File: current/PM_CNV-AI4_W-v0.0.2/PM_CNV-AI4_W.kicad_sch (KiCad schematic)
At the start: 71 parts, among them J1 AFA07-S10FCC-00, J4 15EDGRHC-THR-3.5-14P, J5 15EDGRHC-THR-3.5-14P, U1 AD7190BRUZ, U2 AD7190BRUZ, U3 CA-IS3761HW, U4 CA-IS3105W

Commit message: PM_CNV-AI4_W-v0.0.2
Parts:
- removed C10, C4: 10 uF, kicad_inventree_lib:TAJA_AVX-M, symbol kicad_inventree_lib:TAJA106M016RNJ
- removed C12, C37: 10uF, Capacitor_SMD:C_0603_1608Metric, symbol kicad_inventree_lib:C_10uF_16V_0603_MLCC-X5R
- removed C2, C8: 100nF, Capacitor_SMD:C_0603_1608Metric, symbol kicad_inventree_lib:C_100nF_16V_0603_MLCC-X7R
- removed C22, C24, C31, C33, C34, C36: 10nF, Capacitor_SMD:C_0603_1608Metric, symbol kicad_inventree_lib:C_10nF_16V_0603_MLCC-X7R
- removed C23, C32, C35: 1uF, Capacitor_SMD:C_0603_1608Metric, symbol kicad_inventree_lib: C_1uF_16V_0603_MLCC-X7R
- removed J1: AFA07-S10FCC-00, kicad_inventree_lib:CONN10_AFA07-S10_JUS, symbol kicad_inventree_lib:AFA07-S10FCC-00
- removed JP5, JP6, JP7, JP8: SolderJumper_2_Open, Jumper:SolderJumper-2_P1.3mm_Open_RoundedPad1.0x1.5mm, symbol Jumper:SolderJumper_2_Open
- removed R10: 10k, Resistor_SMD:R_0603_1608Metric, symbol kicad_inventree_lib:R_10k_0603_1%
- removed U1, U2: AD7190BRUZ, kicad_inventree_lib:RU_24_ADI-M, symbol kicad_inventree_lib:AD7190BRUZ
- removed U3: CA-IS3761HW, kicad_inventree_lib:SOIC16-WBW_CLG-M, symbol kicad_inventree_lib:CA-IS3761HW
- added C12, C37: 10uF, Capacitor_SMD:C_0805_2012Metric, symbol kicad_inventree_lib:C_10uF_16V_0805_MLCC-X7R
- added D1, D2, D3: XL-1606SYGC, kicad_inventree_lib:XL-1606, symbol kicad_inventree_lib:XL-1606SYGC
- added D17, D18: XL-1606UBC, kicad_inventree_lib:XL-1606, symbol kicad_inventree_lib:XL-1606UBC
- added D4, D5: XL-1606SURC, kicad_inventree_lib:XL-1606, symbol kicad_inventree_lib:XL-1606SURC
- added J1: FFC_12P_P1.0_100mm_straight, symbol kicad_inventree_lib:FFC_12P_P1.0_100mm_straight
- added J2, J6, J7: AFA07-S12FCC-00, kicad_inventree_lib:CONN10_AFA07-S12_JUS, symbol kicad_inventree_lib:AFA07-S12FCC-00
- added J3: FFC_10P_P1.0_50mm_reverse, symbol kicad_inventree_lib:FFC_10P_P1.0_50mm_reverse
- added R10, R12, R13, R14, R15, R16, R17: 1k, Resistor_SMD:R_0603_1608Metric, symbol kicad_inventree_lib:R_1k_0603_1%
- added SP1: ~, kicad_inventree_lib:PM_LED-xx-v0.0.1, symbol kicad_inventree_lib:PM_LED-10-v0.0.1
- added U1, U2: 5117, kicad_inventree_lib:5117, symbol kicad_inventree_lib:5117
- added U5: SN74LVC2G14DBVR, kicad_inventree_lib:DBV6-M, symbol kicad_inventree_lib:SN74LVC2G14DBVR
- added U6: ~, kicad_inventree_lib:PM-ESP32C3_v0.0.5, symbol kicad_inventree_lib:PM-ESP32C3_v0.0.5
- added U7: AD7193BRUZ, kicad_inventree_lib:RU_28_ADI, symbol kicad_inventree_lib:AD7193BRUZ
- added U8: CA-IS3741HW, kicad_inventree_lib:SOIC16-WBW_CLG-M, symbol kicad_inventree_lib:CA-IS3741HW
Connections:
- net 1.SENSE+ is gone; now on net SENSE+: J4.12 (Pin_10)
- net 1.SENSE- is gone; now on net SENSE-: J4.11 (Pin_8)
- net 2.EXC- is gone; now on net EXC-: J5.13 (Pin_10), J5.6 (Pin_9)
- net 2.SENSE+ is gone; now on net SENSE+: J5.5 (Pin_9)
- net 2.SENSE- is gone; now on net SENSE-: J5.4
- net 3.SENSE+ is gone; now on net SENSE+: J5.12 (Pin_10)
- net 3.SENSE- is gone; now on net SENSE-: J5.11 (Pin_8)
- net CS_MCU: now reaches JP1.2 (B), JP2.2 (B), JP3.2 (B), JP4.2 (B)
- net CS_MCU: now also U8.5 (VI3)
- net CS_CNV: now reaches R11.2
- net CS_CNV: now also U5.3 (2A), U7.4 (CS), U8.12 (VO3)
- net +3.3V renamed +3.3V_MCU
- net +3.3V_MCU: now also J2.10 (Pin_10), J7.3 (Pin_3), U8.1 (VDD), U8.7 (ENA); no longer R11.1
- net +5V renamed +5V_MCU
- net +5V_MCU: now also C12.1, J2.11 (Pin_11), J7.2 (Pin_2)
- net +5V_ISO renamed +5V_CNV
- net +5V_CNV: now also C6.2, R11.1, C37.1, J6.11 (Pin_11), U5.5 (VCC), U7.25 (DVDD), U8.10 (ENB), U8.16 (VISO); no longer C6.1
- net 0.EXC- renamed EXC-
- net EXC-: now also U7.21 (BPDSW)
- net 0.SENSE+ renamed SENSE+
- net SENSE+: now also C19.1, U7.19 (REFIN1(+)); no longer C19.2
- net 0.SENSE- renamed SENSE-
- net SENSE-: now also U7.20 (REFIN1(-))
- net AD_0_AIN0 renamed AIN5
- net AIN5: now also C16.1, U7.15 (AIN5); no longer C16.2
- net AD_0_AIN1 renamed AIN6
- net AIN6: now also U7.16 (AIN6)
- net AD_0_AIN2 renamed AIN7
- net AIN7: now also C13.1, U7.17 (AIN7); no longer C13.2
- net AD_0_AIN3 renamed AIN8
- net AIN8: now also U7.18 (AIN8)
- net AD_1_AIN0 renamed AIN1
- net AIN1: now also C28.1, U7.11 (AIN1); no longer C28.2
- net AD_1_AIN1 renamed AIN2
- net AIN2: now also U7.12 (AIN2)
- net AD_1_AIN2 renamed AIN3
- net AIN3: now also C25.1, U7.13 (AIN3); no longer C25.2
- net AD_1_AIN3 renamed AIN4
- net AIN4: now also U7.14 (AIN4)
- net AGND renamed GND_CNV
- net GND_CNV: now also C13.2, C16.2, C19.2, C25.2, C28.2, C37.2, J6.1 (Pin_1), J6.12 (Pin_11), J6.13 (Pin_11), U1.1, U5.2 (GND), U7.10 (AINCOM), U7.22 (AGND), U7.23 (DGND), U8.15 (GNDB), U8.9 (GNDB); no longer C13.1, C16.1, C19.1, C25.1, C28.1, C6.2
- net AVDD renamed +5V_CNV_FLT
- net +5V_CNV_FLT: now also U7.24 (AVDD)
- net CS0 renamed CS0_MCU
- net CS0_MCU: now also J2.6 (Pin_6), J7.7 (Pin_7)
- net CS1 renamed CS1_MCU
- net CS1_MCU: now also J2.5 (Pin_5), J7.8 (Pin_8)
- net CS2 renamed CS2_MCU
- net CS2_MCU: now also J2.4 (Pin_4), J7.9 (Pin_9)
- net CS3 renamed CS3_MCU
- net CS3_MCU: now also J2.3 (Pin_3), J7.10 (Pin_10)
- net GND renamed GND_MCU
- net GND_MCU: now also C12.2, J2.1 (Pin_1), J2.12 (Pin_11), J2.13 (Pin_11), J7.1 (Pin_1), J7.12 (Pin_11), J7.13 (Pin_11), U2.1, U8.2 (GNDA), U8.8 (GNDA)
- new net: D5.2 (A), R15.2
- new net: D4.2 (A), R14.2
- new net: D18.2 (A), R16.2
- new net: D17.2 (A), R17.2
- new net: D1.2 (A), R10.2
- new net: D3.2 (A), R13.2
- new net: D2.2 (A), R12.2
- new net CS_LED: J6.3 (Pin_3), U5.4 (2Y)
- new net DGND: C6.1
- new net INT_MCU: J2.2 (Pin_2), J7.11 (Pin_11)
- new net MISO_CNV: U5.1 (1A), U7.27 (MISO), U8.11 (VI4)
- new net MISO_LED: J6.2 (Pin_2), U5.6 (1Y)
- new net MISO_MCU: J2.8 (Pin_8), J7.5 (Pin_5), U8.6 (VO4)
- new net MOSI_CNV: U7.28 (MOSI), U8.14 (VO1)
- new net MOSI_MCU: J2.9 (Pin_9), J7.4 (Pin_4), U8.3 (VI1)
- new net P0: J6.7 (Pin_7), U7.8 (P0)
- new net P1: J6.8 (Pin_8), U7.7 (P1)
- new net P2: J6.9 (Pin_9), U7.6 (P2)
- new net P3: J6.10 (Pin_10), U7.5 (P3)
- new net SCK_CNV: U7.3 (SCK), U8.13 (VO2)
- new net SCK_MCU: J2.7 (Pin_7), J7.6 (Pin_6), U8.4 (VI2)
- no-connect marks 15 -> 20
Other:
- removed sheet subplates
- note added: "АЦП"
- note added: "Входные фильтры"
- note added: "Изоляция SPI"
- note added: "Клеммник"
- note added: "Плата светодиодов"
- note removed: "Изменить 10uF тип на X7R - увеличить посадочное место"
- moved on the sheet: C1, C11, C13, C14, C15, C16, C17, C18, C19, C20, C21, C25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

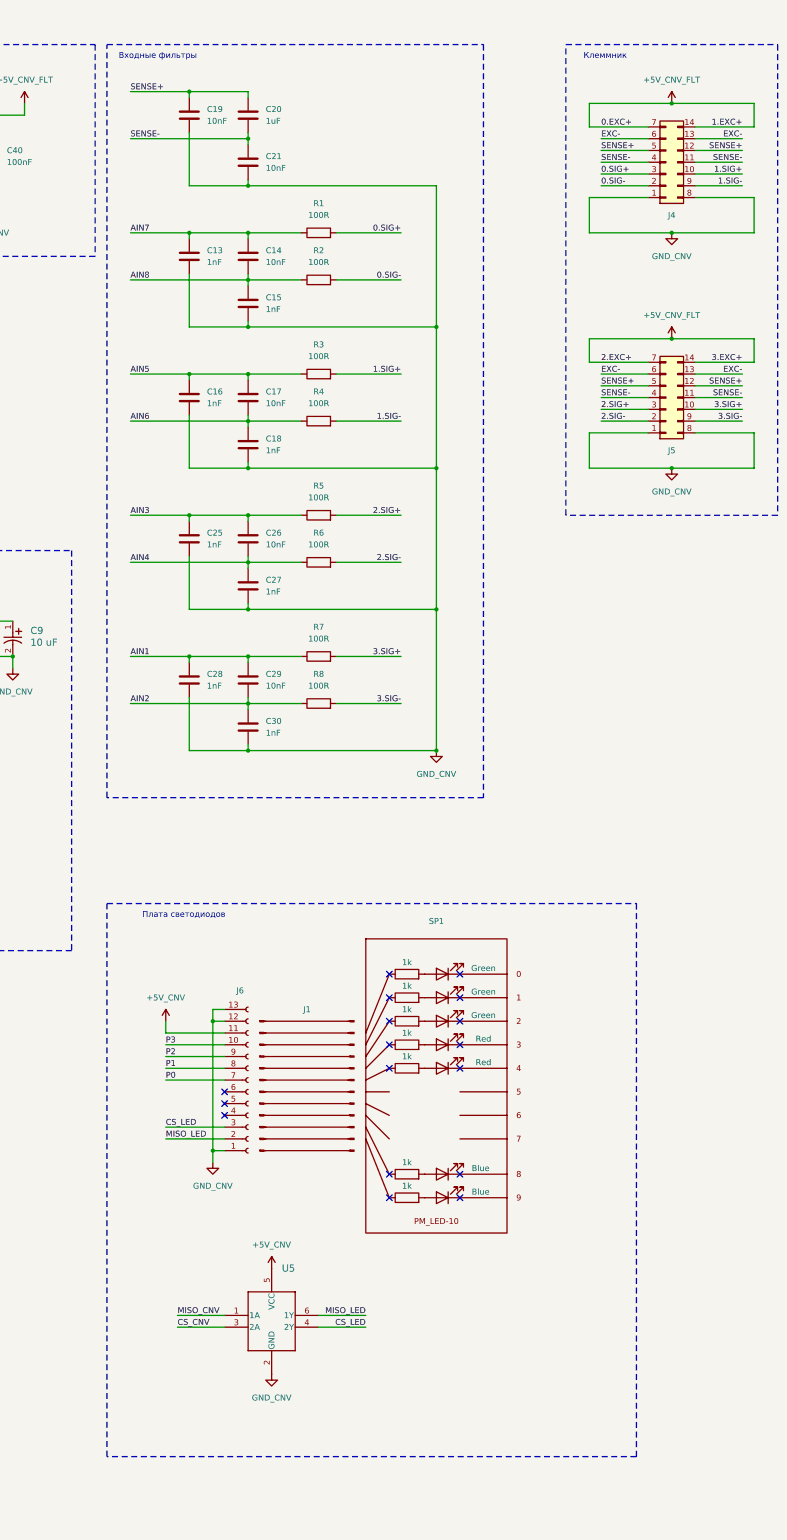
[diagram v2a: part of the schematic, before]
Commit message: nextpcb order
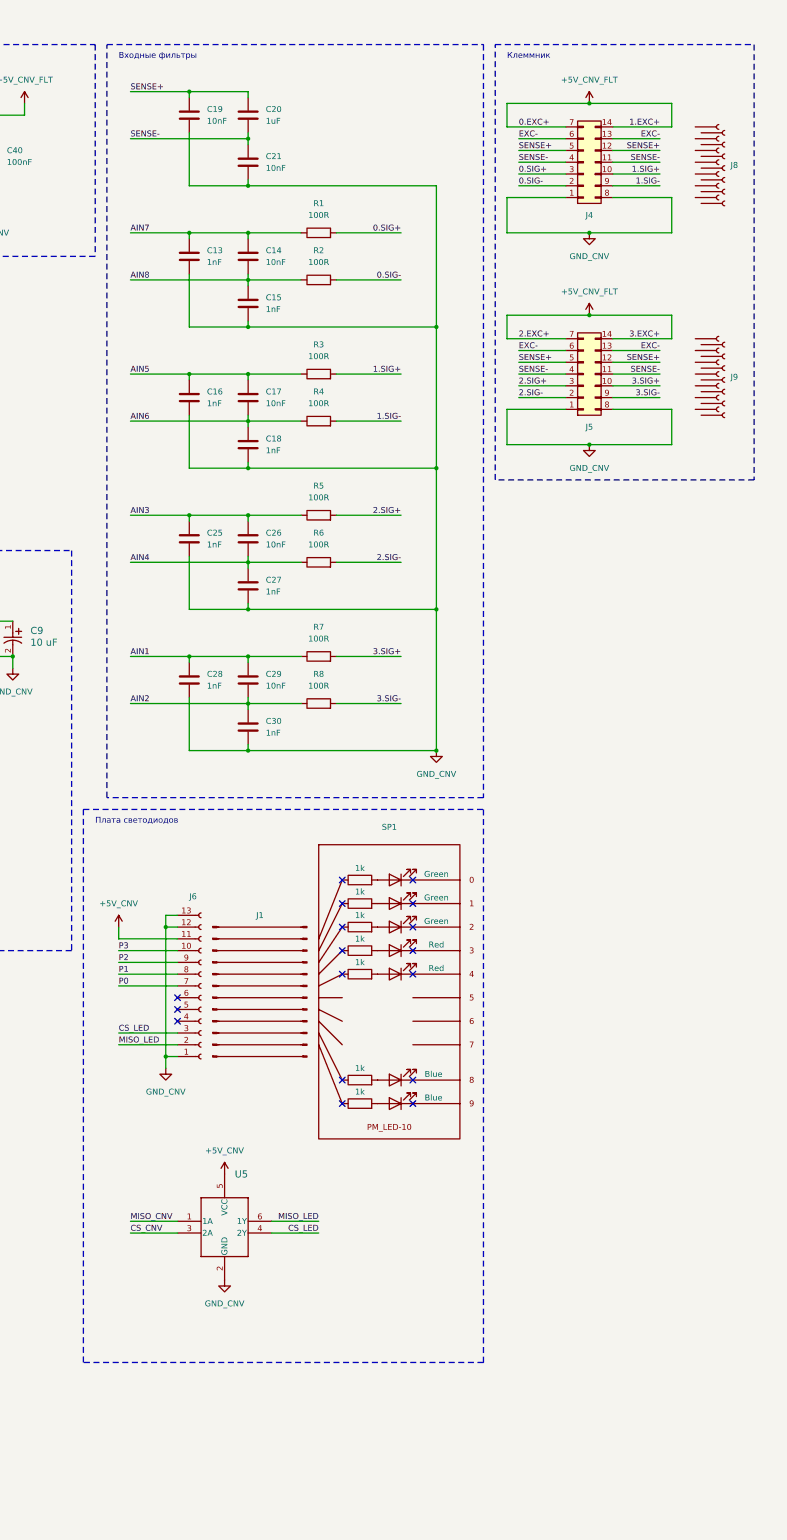
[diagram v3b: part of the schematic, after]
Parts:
- added J8, J9: 15EDGKNH-3.5-14P, symbol kicad_inventree_lib:15EDGKNH-3.5-14P
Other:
- moved on the sheet: J1, J4, J5, J6, SP1, U5
